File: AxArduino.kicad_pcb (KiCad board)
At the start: 2 copper layers, 86 x 33 mm, 40 parts, among them P1 CONN_01X02, P10 CONN_01X04, P11 CONN_01X04, P2 CONN_01X02, P3 CONN_01X03, P4 CONN_01X03, P5 CONN_01X03, P7 CONN_01X03, P8 CONN_01X15, P9 CONN_01X15, U1 MCP2515-I/ST, U2 MCP2551-I-SN, U3 74LS241, Y1 Crystal

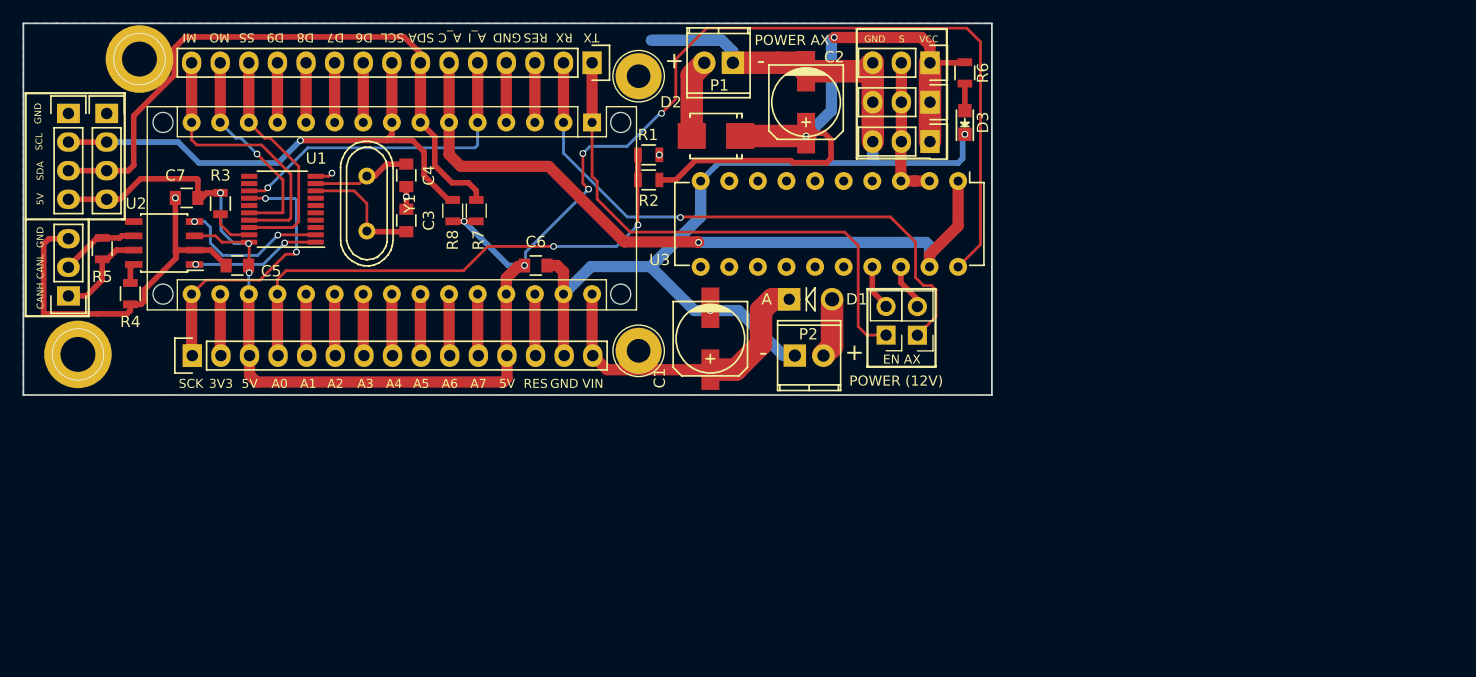
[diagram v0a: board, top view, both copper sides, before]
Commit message: New design
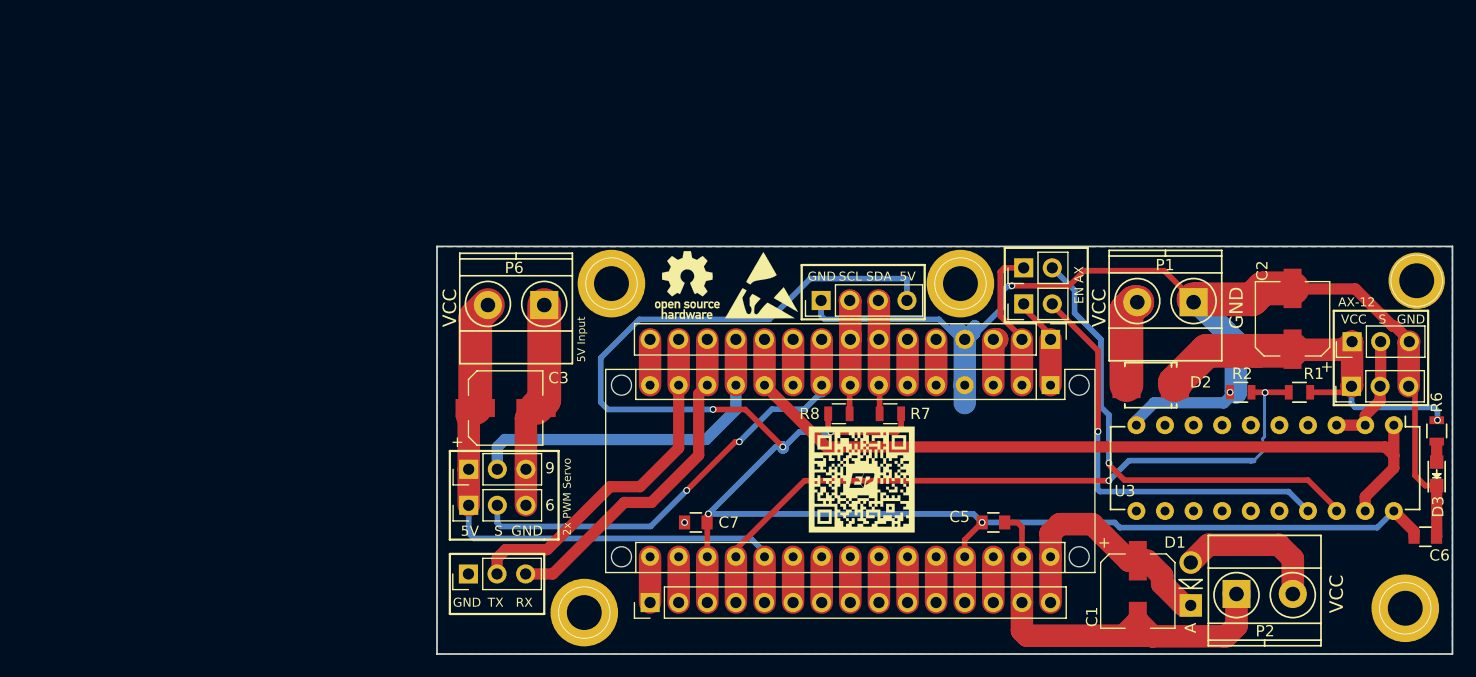
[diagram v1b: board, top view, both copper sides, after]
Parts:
- removed C4: C, Capacitors_SMD:C_0805
- removed the G*** at (118.2, 77.9)
- removed P10: CONN_01X04, Pin_Headers:Pin_Header_Straight_1x04
- removed R3: 10K, Resistors_SMD:R_0805
- removed R4: 4.7K, Resistors_SMD:R_0805
- removed R5: 120, Resistors_SMD:R_0805
- removed the REF** at (53.8, 100.4)
- removed the REF** at (59.3, 74.2)
- removed the REF** at (103.6, 75.7)
- removed the REF** at (103.6, 100.1)
- removed U1: MCP2515-I/ST, Housings_SSOP:TSSOP-20_4.4x6.5mm_Pitch0.65mm
- removed U2: MCP2551-I-SN, Housings_SOIC:SOIC-8_3.9x4.9mm_Pitch1.27mm
- removed Y1: Crystal, Crystals:Crystal_HC49-U_Vertical
- added G***: LOGO, Hardware:EP_Logo, B.Cu at (92.7, 103.4)
- added G***: LOGO, Hardware:EP_Logo, F.Cu at (123.4, 111.5)
- added P12: CONN_01X03, Pin_Headers:Pin_Header_Straight_1x03_Pitch2.54mm, F.Cu at (88.5, 110.6)
- added P6: CONN_01X02, Connectors_Terminal_Blocks:TerminalBlock_Pheonix_MKDS1.5-2pol, F.Cu at (95.2, 96.0)
- added REF**: 1pin, Connectors:1pin, F.Cu at (171.7, 122.9)
- added REF**: 1pin, Connectors:1pin, F.Cu at (172.7, 93.9)
- added REF**: 1pin, Connectors:1pin, F.Cu at (132.2, 94.1)
- added REF**: 1pin, Connectors:1pin, F.Cu at (101.2, 94.1)
- added REF**: 1pin, Connectors:1pin, F.Cu at (98.8, 123.3)
- added REF***: ESD-Logo_6.6x6mm_SilkScreen, Symbols:ESD-Logo_6.6x6mm_SilkScreen, F.Cu at (114.6, 94.2)
- added REF***: OSHW-Logo_5.7x6mm_SilkScreen, Symbols:OSHW-Logo_5.7x6mm_SilkScreen, F.Cu at (108.0, 94.2)
- added REF***: KiCad-Logo2_6mm_SilkScreen, Symbols:KiCad-Logo2_6mm_SilkScreen, B.Cu at (162.8, 94.5)
- C1, C2: footprint Capacitors_SMD:c_elec_6.3x5.3 -> Capacitors_SMD:CP_Elec_6.3x5.3
- C3: value C -> CP; footprint Capacitors_SMD:C_0805 -> Capacitors_SMD:CP_Elec_6.3x5.3
- P1, P2: footprint Terminal_Blocks:TerminalBlock_Pheonix_MPT-2.54mm_2pol -> Connectors_Terminal_Blocks:TerminalBlock_Pheonix_MKDS1.5-2pol
- P11: footprint Pin_Headers:Pin_Header_Straight_1x04 -> Pin_Headers:Pin_Header_Straight_1x04_Pitch2.54mm
- P3, P4, P5, P7: footprint Pin_Headers:Pin_Header_Straight_1x03 -> Pin_Headers:Pin_Header_Straight_1x03_Pitch2.54mm
- P8, P9: footprint Pin_Headers:Pin_Header_Straight_1x15 -> Pin_Headers:Pin_Header_Straight_1x15_Pitch2.54mm
- moved C6 82.6 mm to (173.5, 116.6)
- moved C5 70.9 mm to (135.1, 115.3), turned to 0 degrees
- moved P11 65.6 mm to (119.8, 95.6), turned to 90 degrees
- moved P5 61.2 mm to (88.5, 119.9), turned to 90 degrees
- moved R1 60.8 mm to (162.3, 103.8)
- moved R2 56.6 mm to (157.1, 103.8), turned to 180 degrees
- moved C7 53.6 mm to (108.7, 115.3)
- moved R6 52.6 mm to (174.5, 107.2)
- moved D3 52.2 mm to (174.5, 111.0)
- moved P8 47.5 mm to (140.2, 99.1)
- moved C2 47.3 mm to (161.7, 97.2), turned to 90 degrees
- moved A1 46.9 mm to (140.2, 103.1)
- moved P9 46.2 mm to (104.6, 122.4)
- moved P1 46.1 mm to (152.9, 95.8)
- moved D1 44.8 mm to (152.7, 122.7), turned to 90 degrees
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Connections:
- A1 pad 11: A_D8 -> A_CONTROL
- A1 pad 6: A_CONTROL -> A_D3
- C3 pad 1: Net-(C3-Pad1) -> A_A1
- P5 pad 1: AX_P -> GND
- P5 pad 2: AX_S -> A_MOSI
- P5 pad 3: GND -> A_SS
- P7 pad 1: Net-(P7-Pad1) -> A_A1
- P7 pad 2: Net-(P7-Pad2) -> A_D6
- P8 pad 11: A_D8 -> A_CONTROL
- P8 pad 6: A_CONTROL -> A_D3
- U3 pad 11: Net-(U3-Pad11) -> (no net)
- U3 pad 12: Net-(U3-Pad12) -> (no net)
- U3 pad 13: Net-(U3-Pad13) -> (no net)
- U3 pad 14: Net-(U3-Pad14) -> (no net)
- U3 pad 15: Net-(U3-Pad15) -> (no net)
- U3 pad 16: Net-(U3-Pad16) -> (no net)
- U3 pad 4: Net-(U3-Pad4) -> (no net)
- U3 pad 5: Net-(U3-Pad5) -> (no net)
- U3 pad 6: Net-(U3-Pad6) -> (no net)
- U3 pad 7: Net-(U3-Pad7) -> (no net)
- U3 pad 8: Net-(U3-Pad8) -> (no net)
- U3 pad 9: Net-(U3-Pad9) -> (no net)
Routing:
- net A_A1: track 5.57 -> 53.4 mm
- net A_SDA: track 56.7 -> 10.1 mm
- net A_RX: track 52.7 -> 13.1 mm, vias 1 -> 0
- net A_TX: track 47.2 -> 8.20 mm
- net A_LS_RX: track 4.29 -> 41.6 mm, vias 0 -> 1
- net A_SCL: track 46.3 -> 10.5 mm, vias 1 -> 0
- net A_D6: track 5.30 -> 40.7 mm, vias 0 -> 2
- net A_LS_TX: track 4.03 -> 37.9 mm, vias 0 -> 1
- net A_D9: track 5.30 -> 30.8 mm
- net A_INT: track 29.3 -> 4.06 mm, vias 1 -> 0
- net AX_P: track 62.7 -> 38.9 mm, vias 2 -> 1
- net GND: track 148.7 -> 172.1 mm, vias 6 -> 3
- net A_SCK: track 25.3 -> 4.06 mm, vias 2 -> 0
- net A_MISO: track 24.6 -> 4.06 mm
- net A_A0: track 47.1 -> 63.8 mm
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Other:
- board size 86 x 33 mm -> 90.2 x 36.2 mm
- board text added: "2x PWM Servo"
- board text added: "5V Input"
- board text added: "6"
- board text added: "9"
- board text added: "AX-12"
- board text added: "AX-Arduino V1.1 https://github.com/Elektropioneer http://elektropioneer.co.rs"
- board text removed: "+"
- board text removed: "-"
- board text removed: "3V3"
- board text removed: "A0"
- board text removed: "A1"
- board text removed: "A2"
- board text removed: "A3"
- board text removed: "A4"
- board text removed: "A5"
- board text removed: "A6"
- board text removed: "A7"
- board text removed: "AX-12 driver 74LS241"
- board text removed: "A_C"
- board text removed: "A_I"
- board text removed: "CAN"
- board text removed: "CANH"
- board text removed: "CANL"
- board text removed: "D6"
- board text removed: "D7"
- board text removed: "D8"
- board text removed: "D9"
- board text removed: "I2C"
- board text removed: "MI"
- board text removed: "MO"
- board text removed: "POWER (12V)"
- board text removed: "POWER AX"
- board text removed: "RES"
- board text removed: "SCK"
- board text removed: "SS"
- board text removed: "VIN"
- board text removed: "http://elektropioneer.co.rs/ https://github.com/Elektropioneer Arduino_CAN_AX"
